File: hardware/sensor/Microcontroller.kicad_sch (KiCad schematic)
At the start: 20 parts, among them J1 Conn_02x03_Odd_Even, J2 Conn_01x08_Pin, SW1 SW_Push, U2 nRF52810-QFxx, Y1 Crystal, Y2 Crystal

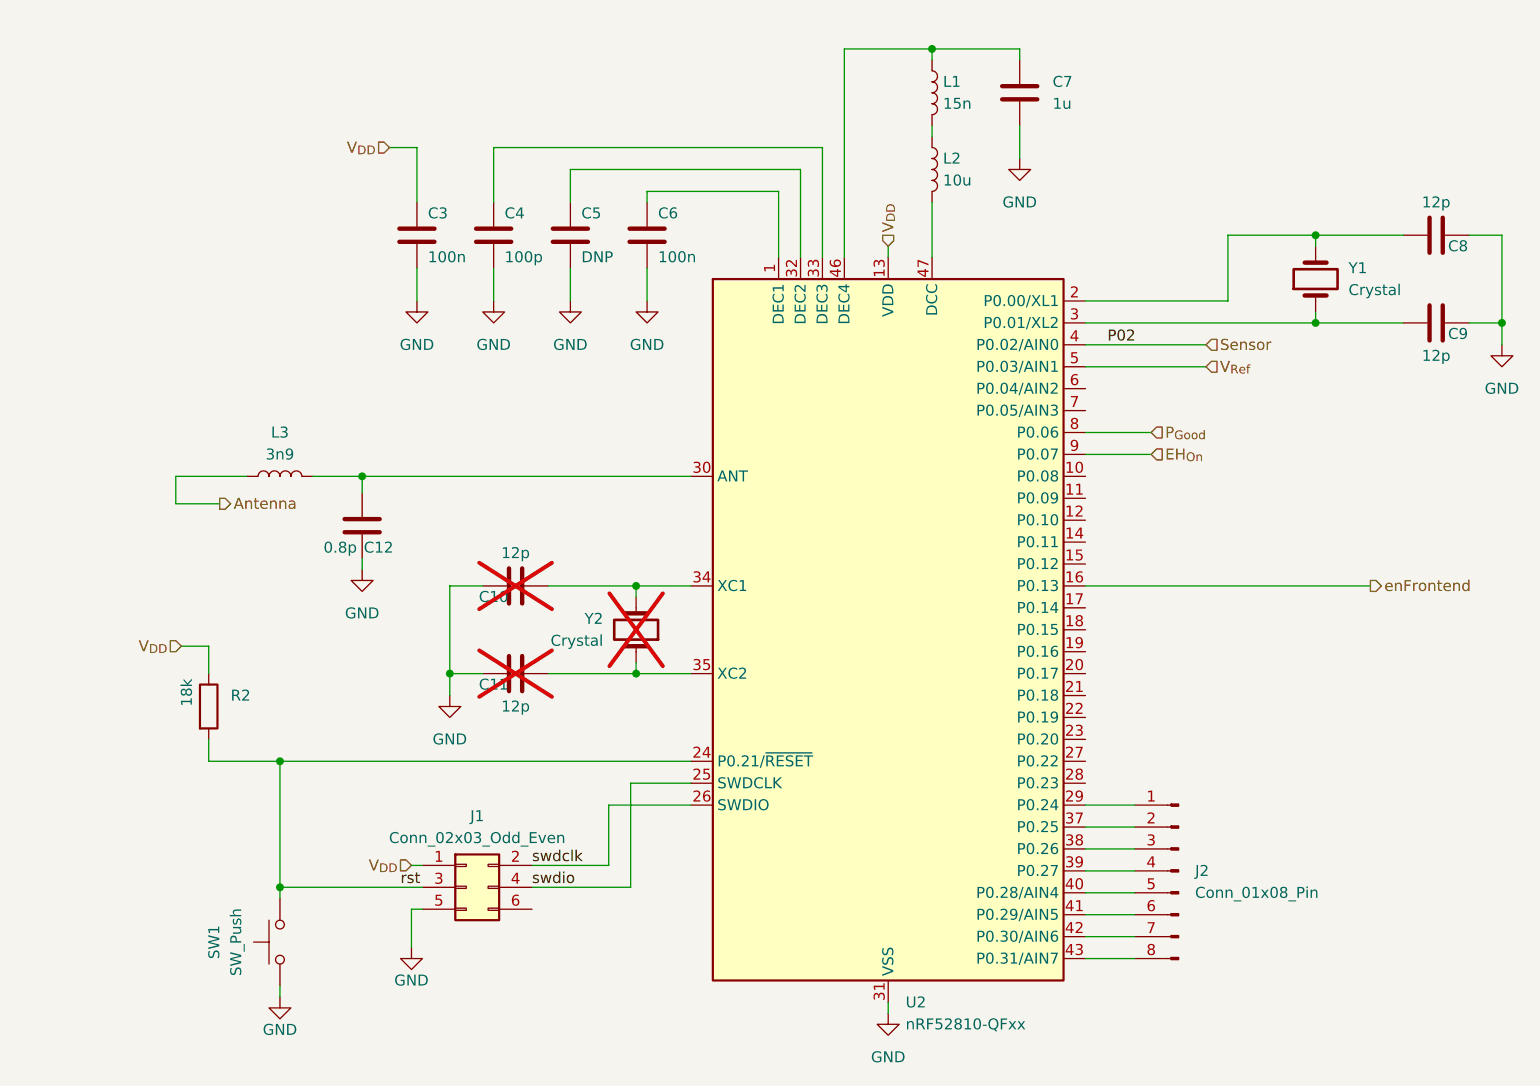
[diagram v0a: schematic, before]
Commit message: Fix incorrect upstream
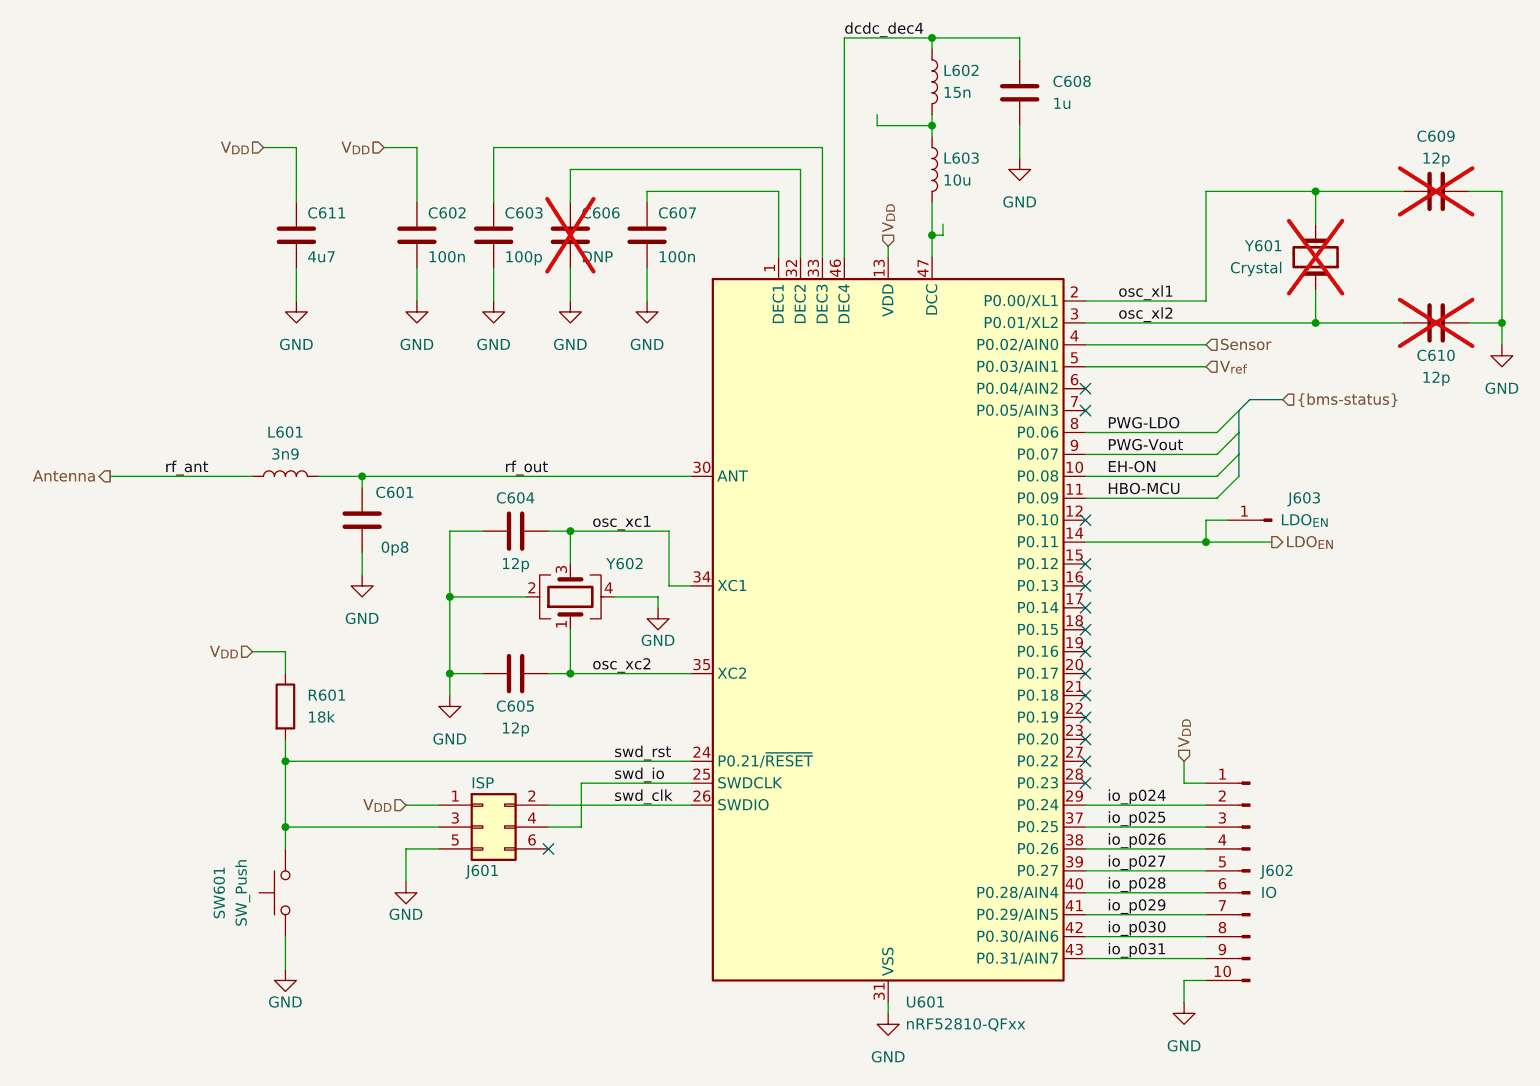
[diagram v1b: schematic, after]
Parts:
- removed J2: Conn_01x08_Pin, symbol Connector:Conn_01x08_Pin
- removed Y1: Crystal, symbol Device:Crystal
- added C611: 4u7, Capacitor_SMD:C_0603_1608Metric_Pad1.08x0.95mm_HandSolder, symbol Device:C
- added J602: IO, Connector_PinHeader_2.54mm:PinHeader_1x10_P2.54mm_Vertical, symbol Connector:Conn_01x10_Pin
- added J603: LDO_{EN}, testpoint_519x:Testpoint_519xTR, symbol Connector:Conn_01x01_Pin
- added Y602: Crystal_GND24, Crystal:Crystal_SMD_2016-4Pin_2.0x1.6mm, symbol Device:Crystal_GND24
- C601: renamed from C12; value 0.8p -> 0p8; footprint (none) -> Capacitor_SMD:C_0402_1005Metric_Pad0.74x0.62mm_HandSolder
- C602: renamed from C3; footprint (none) -> Capacitor_SMD:C_0402_1005Metric_Pad0.74x0.62mm_HandSolder
- C603: renamed from C4; footprint (none) -> Capacitor_SMD:C_0402_1005Metric_Pad0.74x0.62mm_HandSolder
- C604: renamed from C10; footprint (none) -> Capacitor_SMD:C_0402_1005Metric_Pad0.74x0.62mm_HandSolder; now fitted
- C605: renamed from C11; footprint (none) -> Capacitor_SMD:C_0402_1005Metric_Pad0.74x0.62mm_HandSolder; now fitted
- C606: renamed from C5; footprint (none) -> Capacitor_SMD:C_0402_1005Metric_Pad0.74x0.62mm_HandSolder; now not fitted
- C607: renamed from C6; footprint (none) -> Capacitor_SMD:C_0402_1005Metric_Pad0.74x0.62mm_HandSolder
- C608: renamed from C7; footprint (none) -> Capacitor_SMD:C_0603_1608Metric_Pad1.08x0.95mm_HandSolder
- C609: renamed from C8; footprint (none) -> Capacitor_SMD:C_0402_1005Metric_Pad0.74x0.62mm_HandSolder; now not fitted
- C610: renamed from C9; footprint (none) -> Capacitor_SMD:C_0402_1005Metric_Pad0.74x0.62mm_HandSolder; now not fitted
- J601: renamed from J1; value Conn_02x03_Odd_Even -> ISP; footprint (none) -> Connector:Tag-Connect_TC2030-IDC-NL_2x03_P1.27mm_Vertical
- L601: renamed from L3; footprint (none) -> Inductor_SMD:L_0402_1005Metric_Pad0.77x0.64mm_HandSolder
- L602: renamed from L1; footprint (none) -> Inductor_SMD:L_0402_1005Metric_Pad0.77x0.64mm_HandSolder
- L603: renamed from L2; footprint (none) -> Inductor_SMD:L_0603_1608Metric_Pad1.05x0.95mm_HandSolder
- R601: renamed from R2; footprint (none) -> Resistor_SMD:R_0805_2012Metric_Pad1.20x1.40mm_HandSolder
- SW601: renamed from SW1; footprint (none) -> Button_Switch_SMD:SW_SPST_B3SL-1002P
- Y601: renamed from Y2; footprint (none) -> Crystal:Crystal_SMD_3215-2Pin_3.2x1.5mm
- renumbered U2 to U601
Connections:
- net GND: now also C611.2, J602.10 (Pin_10), Y602.2, Y602.4
- net V_{DD}: now also C611.1, J602.1 (Pin_1)
- net osc_xl2: now reaches C610.1, U601.3 (P0.01/XL2)
- net osc_xl2: now also Y601.1
- net osc_xl1: now reaches C609.1, U601.2 (P0.00/XL1)
- net osc_xl1: now also Y601.2
- net dcdc_dec4: now reaches C608.1, L602.1, U601.46 (DEC4)
- net rf_out: now reaches C601.1, L601.2, U601.30 (ANT)
- net osc_xc1: now reaches C604.1, U601.34 (XC1)
- net osc_xc1: now also Y602.3; no longer Y601.2
- net io_p024: now reaches U601.29 (P0.24)
- net io_p024: now also J602.2 (Pin_2)
- net io_p025: now reaches U601.37 (P0.25)
- net io_p025: now also J602.3 (Pin_3)
- net io_p026: now reaches U601.38 (P0.26)
- net io_p026: now also J602.4 (Pin_4)
- net io_p027: now reaches U601.39 (P0.27)
- net io_p027: now also J602.5 (Pin_5)
- net io_p028: now reaches U601.40 (P0.28/AIN4)
- net io_p028: now also J602.6 (Pin_6)
- net io_p029: now reaches U601.41 (P0.29/AIN5)
- net io_p029: now also J602.7 (Pin_7)
- net io_p030: now reaches U601.42 (P0.30/AIN6)
- net io_p030: now also J602.8 (Pin_8)
- net io_p031: now reaches U601.43 (P0.31/AIN7)
- net io_p031: now also J602.9 (Pin_9)
- net osc_xc2: now reaches C605.1, U601.35 (XC2)
- net osc_xc2: now also Y602.1; no longer Y601.1
- net EH-ON: now reaches U601.10 (P0.08)
- net HBO-MCU: now reaches U601.11 (P0.09)
- net LDO_{EN}: now reaches U601.14 (P0.11)
- net LDO_{EN}: now also J603.1 (Pin_1)
- net EH_{On} renamed PWG-Vout
- net P_{Good} renamed PWG-LDO
- net V_{Ref} renamed V_{ref}
- net enFrontend: no longer names the net of U601.16 (P0.13)
- net rst renamed swd_rst
- net swdclk renamed swd_clk
- net swdio renamed swd_io
- no-connect marks 0 -> 15
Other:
- moved on the sheet: C601, J601, L601, L602, R601, SW601, Y601
